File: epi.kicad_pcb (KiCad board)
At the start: 4 copper layers, 12.7 x 22.8 mm, 36 parts, among them J1 Connector 1x12, J2 Connector 1x12, J3 Conn_01x05, J4 USB-C 2.0 mid-mount female co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, U1 ATmega32U4-M, Y1 Crystal_GND24

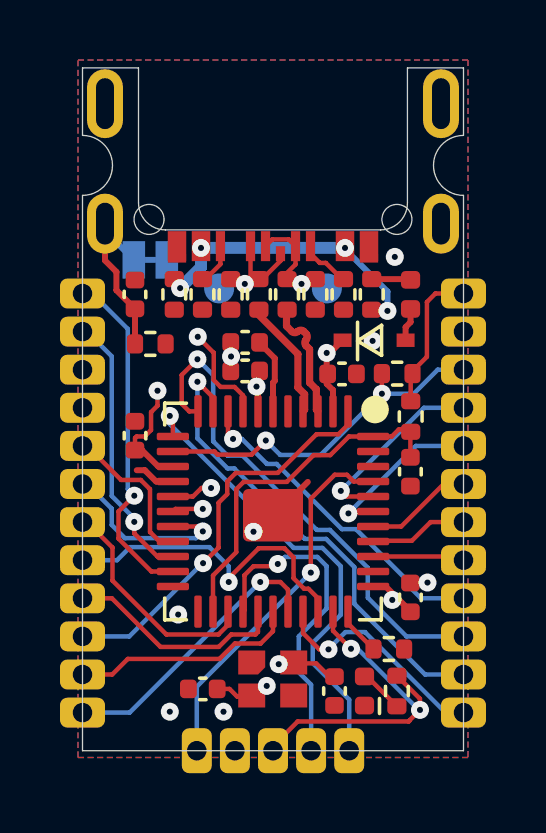
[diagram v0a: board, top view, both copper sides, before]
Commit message: big redesign
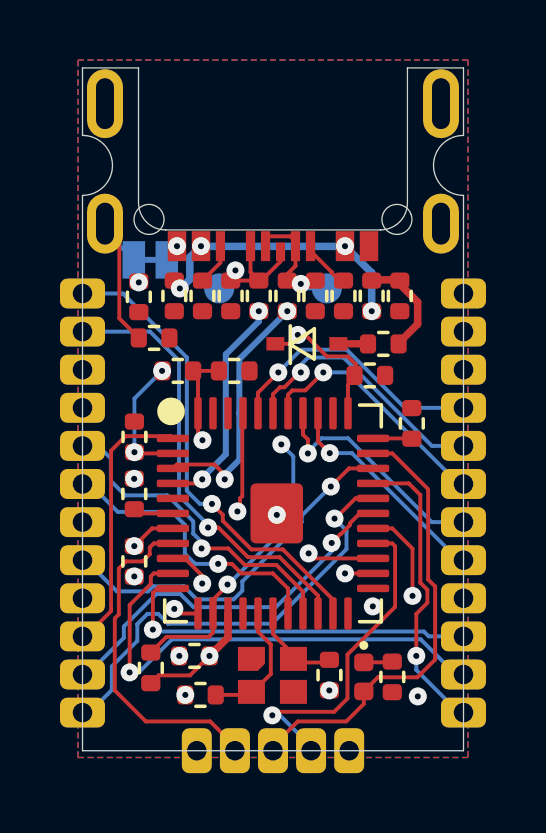
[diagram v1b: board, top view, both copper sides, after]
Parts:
- added C7: 10µF, Resistor_SMD:R_0402_1005Metric, F.Cu at (108.5, 59.0)
- C1, C10, C2, C3, C4, C5, C6, C8, C9: footprint Capacitor_SMD:C_0402_1005Metric -> Resistor_SMD:R_0402_1005Metric
- F1: footprint Fuse:Fuse_0402_1005Metric -> Resistor_SMD:R_0402_1005Metric
- moved R6 12.8 mm to (100.2, 71.4), turned to 90 degrees
- moved R9 7.91 mm to (101.1, 61.5), turned to 0 degrees
- moved R7 7.56 mm to (108.9, 63.2), turned to 90 degrees
- moved C3 7.46 mm to (101.7, 71.0), turned to 0 degrees
- moved C4 7.35 mm to (99.7, 67.8), turned to -90 degrees
- moved C2 6.77 mm to (103.0, 61.5), turned to 180 degrees
- moved C8 6.26 mm to (99.7, 65.6), turned to -90 degrees
- moved D2 2.25 mm to (105.4, 60.6)
- moved F1 1.88 mm to (108.0, 60.6), turned to 180 degrees
- moved C10 0.93 mm to (107.5, 61.6)
- moved C5 0.56 mm to (106.2, 71.6)
- moved R8 0.49 mm to (108.2, 71.7)
- moved D1 0.47 mm to (107.3, 71.7), turned to -90 degrees
- moved R3 0.24 mm to (100.3, 60.4)
- moved C6 0.21 mm to (101.9, 72.3)
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- renumbered REF** to DRILL1, REF** to DRILL2
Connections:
- D1 pad 1: GND -> Net-(D1-K)
- D1 pad 2: Net-(D1-A) -> D13
- R8 pad 1: D13 -> Net-(D1-K)
- R8 pad 2: Net-(D1-A) -> GND
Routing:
- net D17/SS: track 19.3 -> 11.3 mm, vias 1 -> 0
- net Net-(U1-XTAL2): track 11.8 -> 4.35 mm, vias 2 -> 0
- net D6: track 7.40 -> 14.8 mm, vias 0 -> 1
- net D4: track 7.62 -> 14.1 mm, vias 0 -> 1
- net Net-(U1-XTAL1): track 9.35 -> 3.07 mm, vias 2 -> 0
- net D2/SDA: track 5.17 -> 10.9 mm, vias 0 -> 1
- net D0/RX: track 9.14 -> 14.8 mm
- net D9: track 9.49 -> 14.9 mm
- net +5V: track 14.6 -> 19.9 mm, vias 4 -> 5
- net D8: track 7.60 -> 12.7 mm, vias 0 -> 1
- net RST: track 11.9 -> 17.0 mm
- net D11: track 15.7 -> 10.7 mm
- net A0: track 3.06 -> 7.88 mm, vias 0 -> 1
- net A2: track 3.60 -> 8.32 mm, vias 0 -> 1
- net A1: track 3.28 -> 7.99 mm, vias 0 -> 1
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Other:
- board text added: "Epi v1,3,0"
- board text removed: "Epi v1,2,4"

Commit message: little fix and updated gerbers
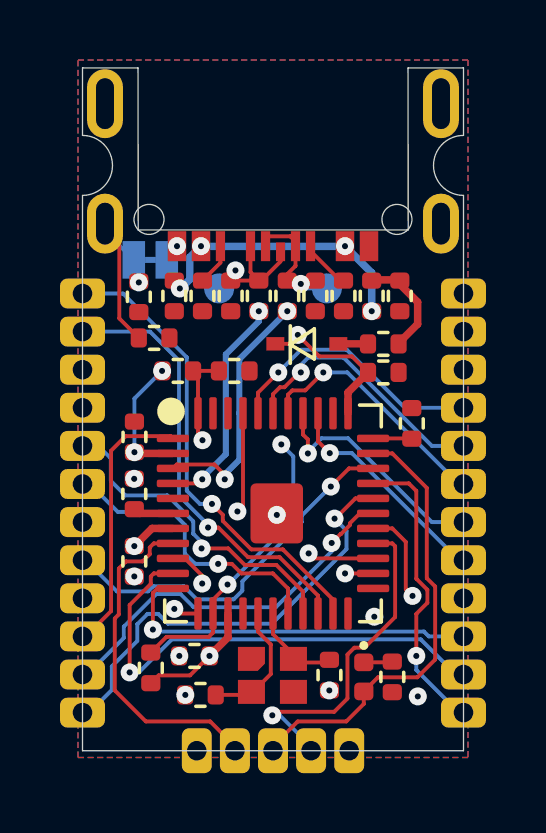
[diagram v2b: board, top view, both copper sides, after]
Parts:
- moved C10 0.46 mm to (108.0, 61.5)
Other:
- outline, holes or cut-outs redrawn
